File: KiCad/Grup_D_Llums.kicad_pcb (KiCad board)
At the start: 2 copper layers, 122.8 x 103.7 mm, 93 parts, among them J1 DE9_Pins, J2 Screw_Terminal_01x02, J3 Screw_Terminal_01x02, J4 Conn_PIC_ICSP_ICD, J5 DE9_Pins, J6 Screw_Terminal_01x02, J7 Conn_01x10_Pin, Q1 AO3400A, Q2 AO3400A, Q3 AO3400A, Q4 AO3400A, Q5 AO3400A, Q6 AO3400A, Q7 AO3400A, Q8 AO3400A, SW1 SW_Push, SW2 SW_SPDT, SW3 SW_SPDT, SW4 SW_SPDT, SW5 SW_SPDT, SW6 SW_SPDT, SW7 SW_SPST, U1 PIC32MX250F128D-IPT, U2 LM2596S-5, U3 L298N, U6 SN65HVD232, U7 LM1117DT-3.3, U9 RPR-0521RS, Y2 Crystal

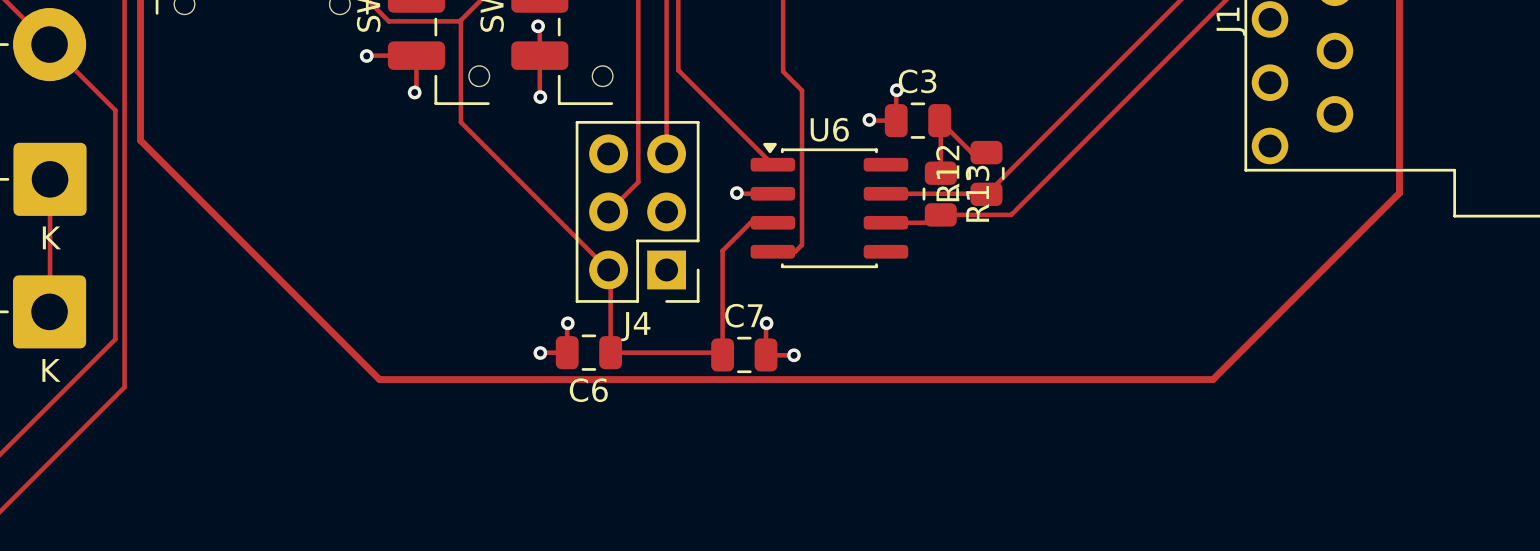
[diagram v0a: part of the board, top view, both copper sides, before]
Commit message: Ayuda
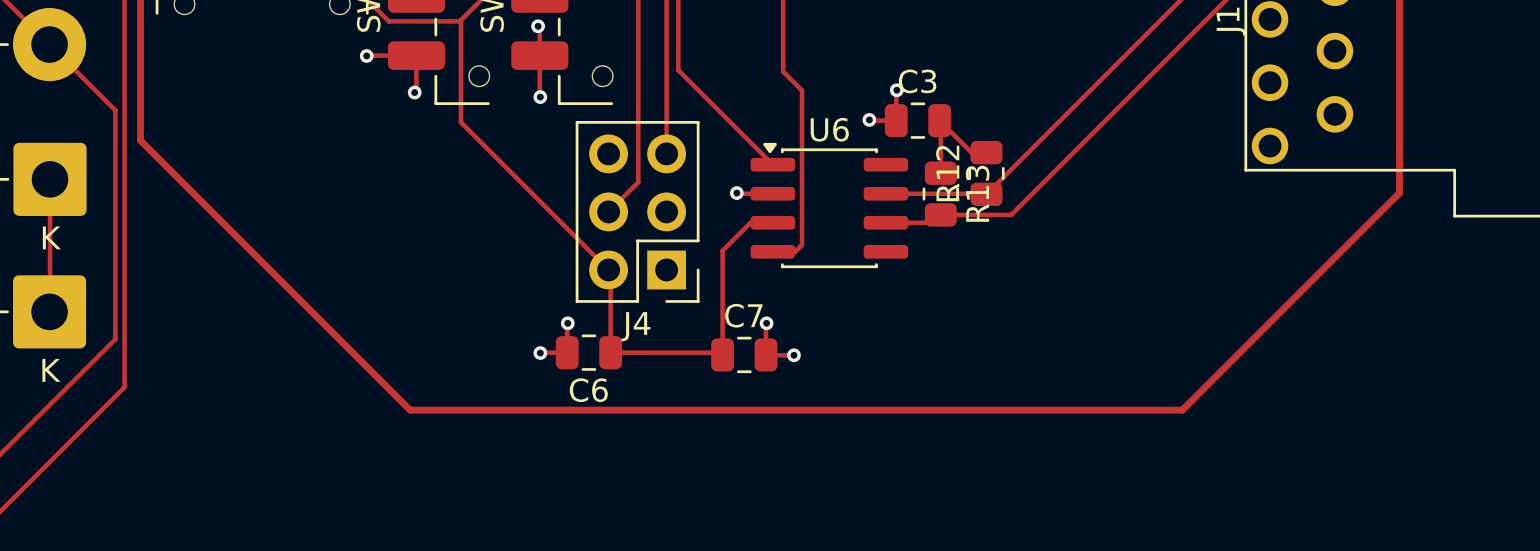
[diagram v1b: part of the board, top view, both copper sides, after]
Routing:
- net VBAT: track 237.6 -> 238.7 mm
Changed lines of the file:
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@@
 		(layer "Edge.Cuts")
 	)
+	(dimension
+		(type orthogonal)
+		(layer "Edge.Cuts")
+		(pts
+			(xy 200.5 53) (xy 200.5 156.7)
+		)
+		(height 19.5)
+		(orientation 1)
+		(format
+			(prefix "")
+			(suffix "")
+			(units 3)
+			(units_format 0)
+			(precision 4)
+			(suppress_zeroes yes)
+		)
+		(style
+			(thickness 0.05)
+			(arrow_length 1.27)
+			(text_position_mode 0)
+			(arrow_direction outward)
+			(extension_height 0.58642)
+			(extension_offset 0.5)
+			(keep_text_aligned yes)
+		)
+		(gr_text "103,7"
+			(at 218.85 104.85 90)
+			(layer "Edge.Cuts")
+			(effects
+				(font
+					(size 1 1)
+					(thickness 0.15)
+				)
+			)
+		)
+	)
+	(dimension
+		(type orthogonal)
+		(layer "Edge.Cuts")
+		(pts
+			(xy 77.7 53) (xy 200.5 53)
+		)
+		(height -13)
+		(orientation 0)
+		(format
+			(prefix "")
+			(suffix "")
+			(units 3)
+			(units_format 0)
+			(precision 4)
+			(suppress_zeroes yes)
+		)
+		(style
+			(thickness 0.05)
+			(arrow_length 1.27)
+			(text_position_mode 0)
+			(arrow_direction outward)
+			(extension_height 0.58642)
+			(extension_offset 0.5)
+			(keep_text_aligned yes)
+		)
+		(gr_text "122,8"
+			(at 139.1 38.85 0)
+			(layer "Edge.Cuts")
+			(effects
+				(font
+					(size 1 1)
+					(thickness 0.15)
+				)
+			)
+		)
+	)
 	(segment
 		(start 172.8125 57.5125)
@@
 	)
 	(segment
-		(start 149.5385 78.674)
-		(end 148.6125 79.6)
+		(start 119.36 109.9)
+		(end 119.36 104.320818)
 		(width 0.3)
 		(layer "F.Cu")
@@
 	)
 	(segment
-		(start 127.86 71.19)
-		(end 127.845 71.175)
-		(width 0.2)
+		(start 149.5385 78.674)
+		(end 148.6125 79.6)
+		(width 0.3)
 		(layer "F.Cu")
 		(net 12)
@@
 	)
 	(segment
+		(start 150.2 140)
+		(end 184 140)
+		(width 0.3)
+		(layer "F.Cu")
+		(net 12)
+	)
+	(segment
+		(start 127.86 71.19)
+		(end 127.845 71.175)
+		(width 0.2)
+		(layer "F.Cu")
+		(net 12)
+	)
+	(segment
 		(start 149.526 80.5135)
 		(end 148.6125 79.6)
@@
 	)
 	(segment
-		(start 119.36 109.9)
-		(end 119.36 104.320818)
+		(start 184 140)
+		(end 193.5 130.5)
 		(width 0.3)
 		(layer "F.Cu")
@@
 	)
 	(segment
-		(start 182.4 74.8)
-		(end 172.94475 84.25525)
+		(start 120.111818 103.569)
+		(end 124.421 103.569)
 		(width 0.3)
 		(layer "F.Cu")
@@
 	)
 	(segment
-		(start 190.6 74.8)
-		(end 182.4 74.8)
-		(width 0.3)
-		(layer "F.Cu")
-		(net 12)
-	)
-	(segment
 		(start 148.525 58.2)
 		(end 149.5365 59.2115)
@@
 	)
 	(segment
-		(start 185.339 138.661)
-		(end 193.5 130.5)
+		(start 151.89213 87.074)
+		(end 149.526 84.70787)
 		(width 0.3)
 		(layer "F.Cu")
@@
 	)
 	(segment
-		(start 120.111818 103.569)
-		(end 124.421 103.569)
+		(start 149.5385 73.4385)
+		(end 149.5385 78.674)
 		(width 0.3)
 		(layer "F.Cu")
@@
 	)
 	(segment
-		(start 151.89213 87.074)
-		(end 149.526 84.70787)
+		(start 149.526 71.547)
+		(end 148.5865 72.4865)
 		(width 0.3)
 		(layer "F.Cu")
@@
 	)
 	(segment
-		(start 148.861 138.661)
-		(end 185.339 138.661)
+		(start 193.5 77.7)
+		(end 190.6 74.8)
 		(width 0.3)
 		(layer "F.Cu")
@@
 	)
 	(segment
-		(start 149.5385 73.4385)
-		(end 149.5385 78.674)
+		(start 182.4 74.8)
+		(end 172.94475 84.25525)
 		(width 0.3)
 		(layer "F.Cu")
@@
 	)
 	(segment
-		(start 149.526 71.547)
-		(end 148.5865 72.4865)
+		(start 170.126 87.074)
+		(end 151.89213 87.074)
 		(width 0.3)
 		(layer "F.Cu")
@@
 	)
 	(segment
-		(start 138.4 128.2)
-		(end 148.861 138.661)
+		(start 149.5365 59.2115)
+		(end 149.5365 64.1885)
 		(width 0.3)
 		(layer "F.Cu")
@@
 	)
 	(segment
-		(start 170.126 87.074)
-		(end 151.89213 87.074)
+		(start 149.526 84.70787)
+		(end 149.526 80.5135)
 		(width 0.3)
 		(layer "F.Cu")
@@
 	)
 	(segment
-		(start 193.5 77.7)
-		(end 190.6 74.8)
+		(start 148.525 65.2)
+		(end 149.526 66.201)
 		(width 0.3)
 		(layer "F.Cu")
@@
 	)
 	(segment
-		(start 149.5365 59.2115)
-		(end 149.5365 64.1885)
+		(start 190.6 74.8)
+		(end 182.4 74.8)
 		(width 0.3)
 		(layer "F.Cu")
@@
 	)
 	(segment
-		(start 193.5 130.5)
-		(end 193.5 77.7)
+		(start 172.94475 84.25525)
+		(end 170.126 87.074)
 		(width 0.3)
 		(layer "F.Cu")
@@
 	)
 	(segment
-		(start 149.526 84.70787)
-		(end 149.526 80.5135)
-		(width 0.3)
-		(layer "F.Cu")
-		(net 12)
-	)
-	(segment
-		(start 148.525 65.2)
-		(end 149.526 66.201)
+		(start 148.5865 72.4865)
+		(end 149.5385 73.4385)
 		(width 0.3)
 		(layer "F.Cu")
@@
 	)
 	(segment
-		(start 172.94475 84.25525)
-		(end 170.126 87.074)
+		(start 138.4 128.2)
+		(end 150.2 140)
 		(width 0.3)
 		(layer "F.Cu")
@@
 	)
 	(segment
-		(start 148.5865 72.4865)
-		(end 149.5385 73.4385)
+		(start 193.5 130.5)
+		(end 193.5 77.7)
 		(width 0.3)
 		(layer "F.Cu")
